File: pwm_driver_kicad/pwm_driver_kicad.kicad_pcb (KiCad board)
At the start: 2 copper layers, 35 x 35 mm, 10 parts, among them J1 Bornera, Q1 IRF540, U1 NE555P

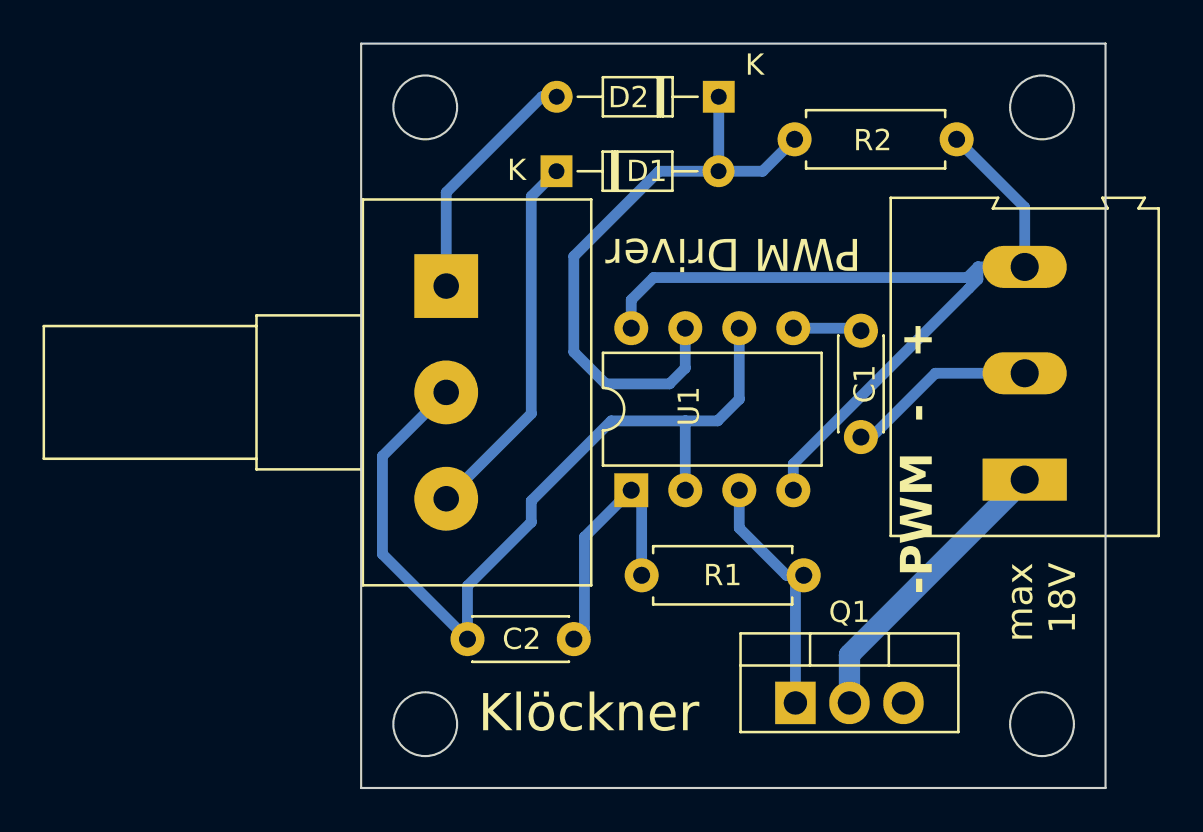
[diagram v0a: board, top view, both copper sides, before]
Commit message: update pcb layout
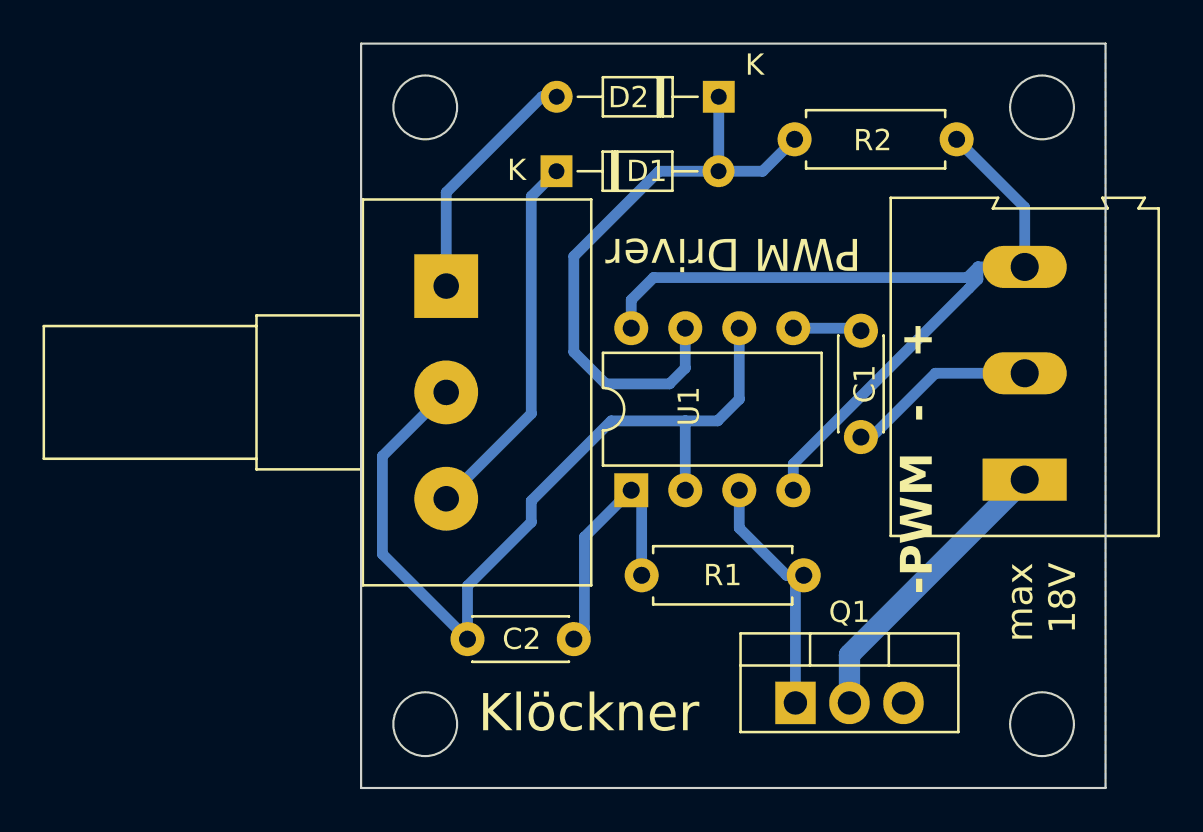
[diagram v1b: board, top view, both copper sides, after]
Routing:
- added copper zone on B.Cu, net GND
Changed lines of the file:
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@@
 		(net 9)
 	)
+	(zone
+		(net 8)
+		(net_name "GND")
+		(layer "B.Cu")
+		(hatch edge 0.5)
+		(connect_pads
+			(clearance 0.5)
+		)
+		(min_thickness 0.25)
+		(filled_areas_thickness no)
+		(fill yes
+			(thermal_gap 0.5)
+			(thermal_bridge_width 0.5)
+		)
+		(polygon
+			(pts
+				(xy 104.9865 45) (xy 139.9865 45) (xy 139.9865 80) (xy 104.9865 80)
+			)
+		)
+	)
 )
